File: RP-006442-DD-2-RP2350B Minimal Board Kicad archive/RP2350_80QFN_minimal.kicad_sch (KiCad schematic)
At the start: 50 parts, among them J1 USB_C_Receptacle_USB2.0_16P, J2 Conn_02x26_Odd_Even, J3 Conn_02x26_Odd_Even, SW1 SW_Push, SW2 SW_Push, U1 RP2350_80QFN, U2 NCP1117-3.3_SOT223, U3 W25Q128JVS, U4 DNF, Y1 ABM8-272-T3

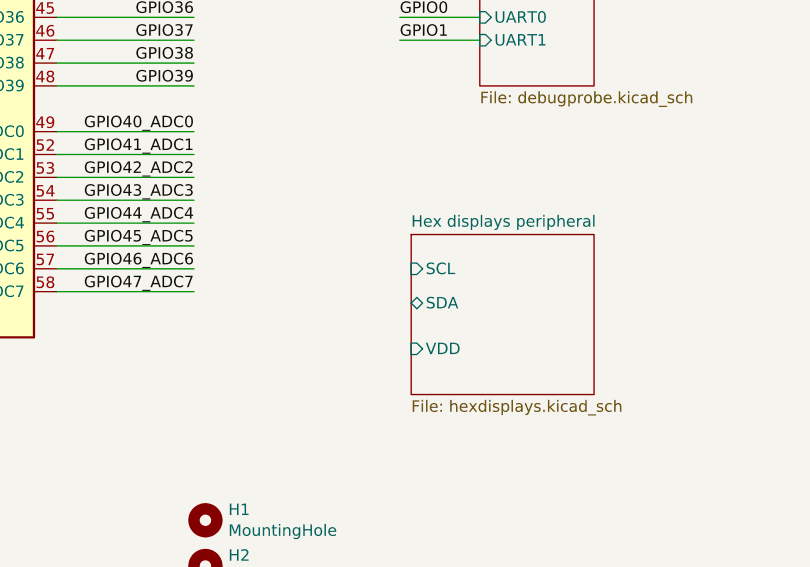
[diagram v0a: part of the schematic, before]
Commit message: Update
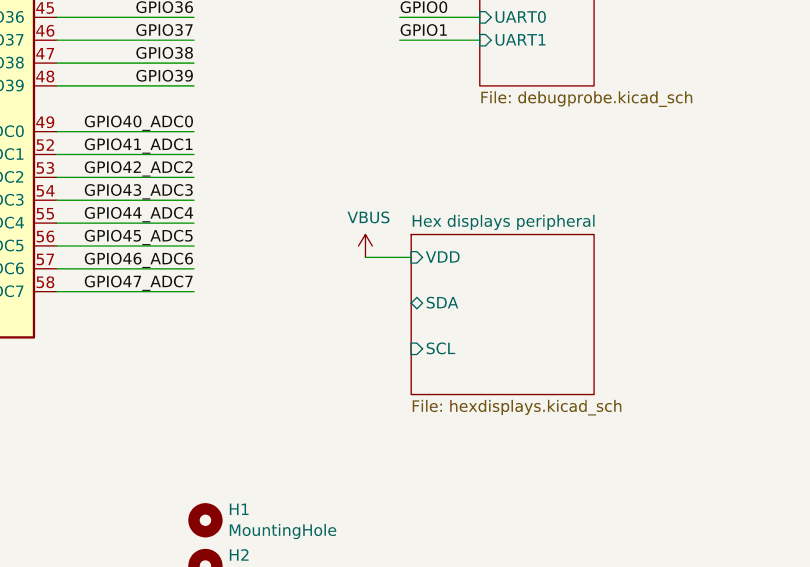
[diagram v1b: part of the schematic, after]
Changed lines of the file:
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@@
 	(wire
 		(pts
+			(xy 269.24 229.87) (xy 274.32 229.87)
+		)
+		(stroke
+			(width 0)
+			(type default)
+		)
+	)
+	(wire
+		(pts
 			(xy 394.97 100.33) (xy 394.97 102.87)
 		)
@@
 	)
 	(symbol
+		(lib_id "power:VBUS")
+		(at 269.24 229.87 0)
+		(unit 1)
+		(exclude_from_sim no)
+		(in_bom yes)
+		(on_board yes)
+		(dnp no)
+		(property "Reference" "#PWR032"
+			(at 269.24 233.68 0)
+			(effects
+				(font
+					(size 1.27 1.27)
+				)
+				(hide yes)
+			)
+		)
+		(property "Value" "VBUS"
+			(at 269.621 225.4758 0)
+			(effects
+				(font
+					(size 1.27 1.27)
+				)
+			)
+		)
+		(property "Footprint" ""
+			(at 269.24 229.87 0)
+			(effects
+				(font
+					(size 1.27 1.27)
+				)
+				(hide yes)
+			)
+		)
+		(property "Datasheet" ""
+			(at 269.24 229.87 0)
+			(effects
+				(font
+					(size 1.27 1.27)
+				)
+				(hide yes)
+			)
+		)
+		(property "Description" ""
+			(at 269.24 229.87 0)
+			(effects
+				(font
+					(size 1.27 1.27)
+				)
+				(hide yes)
+			)
+		)
+		(pin "1"
+		)
+		(instances
+			(project "RP2350_80QFN_minimal"
+				(path "/94683f5c-9cd9-448e-be96-9792537b5cb8"
+					(reference "#PWR032")
+					(unit 1)
+				)
+			)
+		)
+	)
+	(symbol
 		(lib_id "power:GND")
 		(at 66.04 49.53 0)
@@
 		)
 		(pin "SCL" input
-			(at 274.32 231.14 180)
+			(at 274.32 240.03 180)
 			(effects
 				(font
@@
 		)
 		(pin "VDD" input
-			(at 274.32 240.03 180)
+			(at 274.32 229.87 180)
 			(effects
 				(font

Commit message: Update
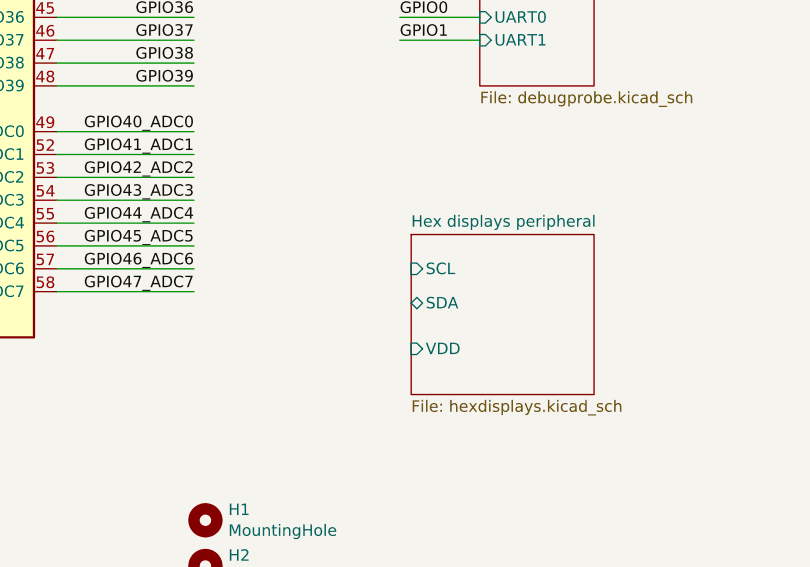
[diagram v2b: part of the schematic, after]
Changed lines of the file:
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@@
 	(wire
 		(pts
-			(xy 269.24 229.87) (xy 274.32 229.87)
-		)
-		(stroke
-			(width 0)
-			(type default)
-		)
-	)
-	(wire
-		(pts
 			(xy 394.97 100.33) (xy 394.97 102.87)
 		)
@@
 	)
 	(symbol
-		(lib_id "power:VBUS")
-		(at 269.24 229.87 0)
-		(unit 1)
-		(exclude_from_sim no)
-		(in_bom yes)
-		(on_board yes)
-		(dnp no)
-		(property "Reference" "#PWR032"
-			(at 269.24 233.68 0)
-			(effects
-				(font
-					(size 1.27 1.27)
-				)
-				(hide yes)
-			)
-		)
-		(property "Value" "VBUS"
-			(at 269.621 225.4758 0)
-			(effects
-				(font
-					(size 1.27 1.27)
-				)
-			)
-		)
-		(property "Footprint" ""
-			(at 269.24 229.87 0)
-			(effects
-				(font
-					(size 1.27 1.27)
-				)
-				(hide yes)
-			)
-		)
-		(property "Datasheet" ""
-			(at 269.24 229.87 0)
-			(effects
-				(font
-					(size 1.27 1.27)
-				)
-				(hide yes)
-			)
-		)
-		(property "Description" ""
-			(at 269.24 229.87 0)
-			(effects
-				(font
-					(size 1.27 1.27)
-				)
-				(hide yes)
-			)
-		)
-		(pin "1"
-		)
-		(instances
-			(project "RP2350_80QFN_minimal"
-				(path "/94683f5c-9cd9-448e-be96-9792537b5cb8"
-					(reference "#PWR032")
-					(unit 1)
-				)
-			)
-		)
-	)
-	(symbol
 		(lib_id "power:GND")
 		(at 66.04 49.53 0)
@@
 		)
 		(pin "SCL" input
-			(at 274.32 240.03 180)
+			(at 274.32 231.14 180)
 			(effects
 				(font
@@
 		)
 		(pin "VDD" input
-			(at 274.32 229.87 180)
+			(at 274.32 240.03 180)
 			(effects
 				(font
